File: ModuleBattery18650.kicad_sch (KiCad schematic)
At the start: 28 parts, among them J1 Connector_6p, T1 SI2323DS-T1-E3, T2 FDN337N, T3 SI2323DS-T1-E3, U1 MCP73832-2-OT, U2 MCP121T-315E

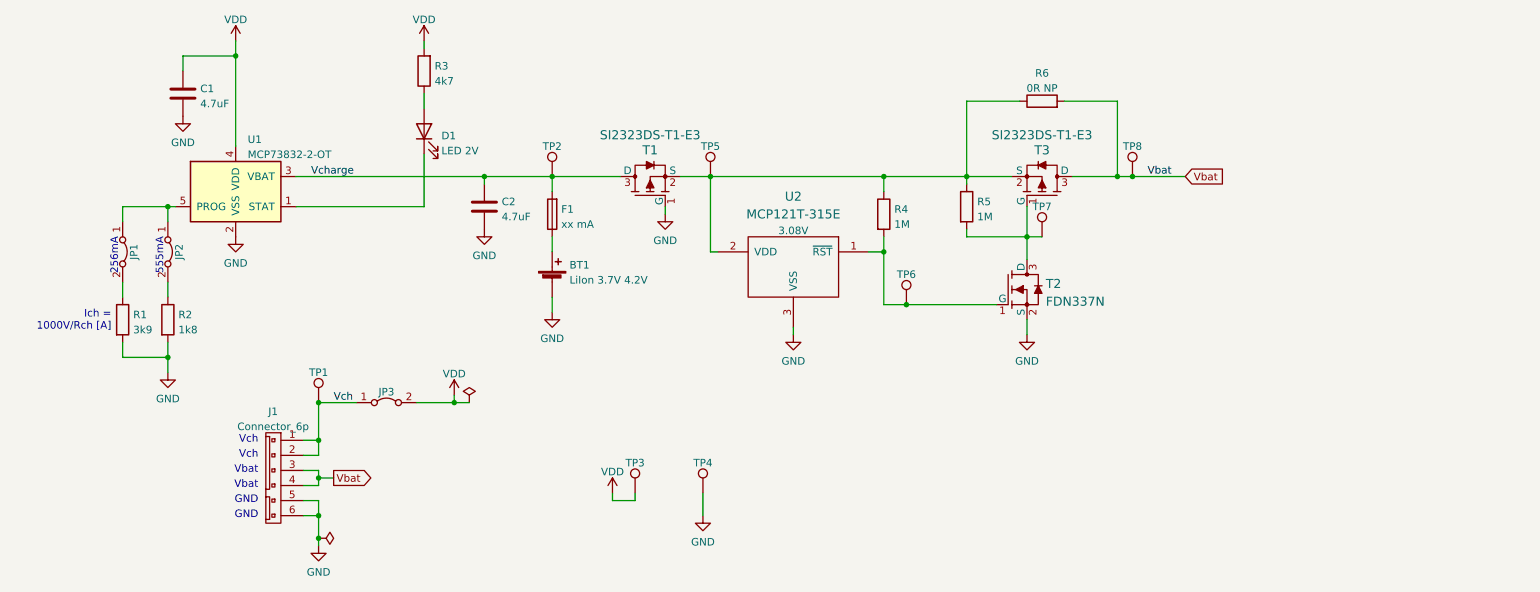
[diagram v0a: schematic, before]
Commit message: Changes
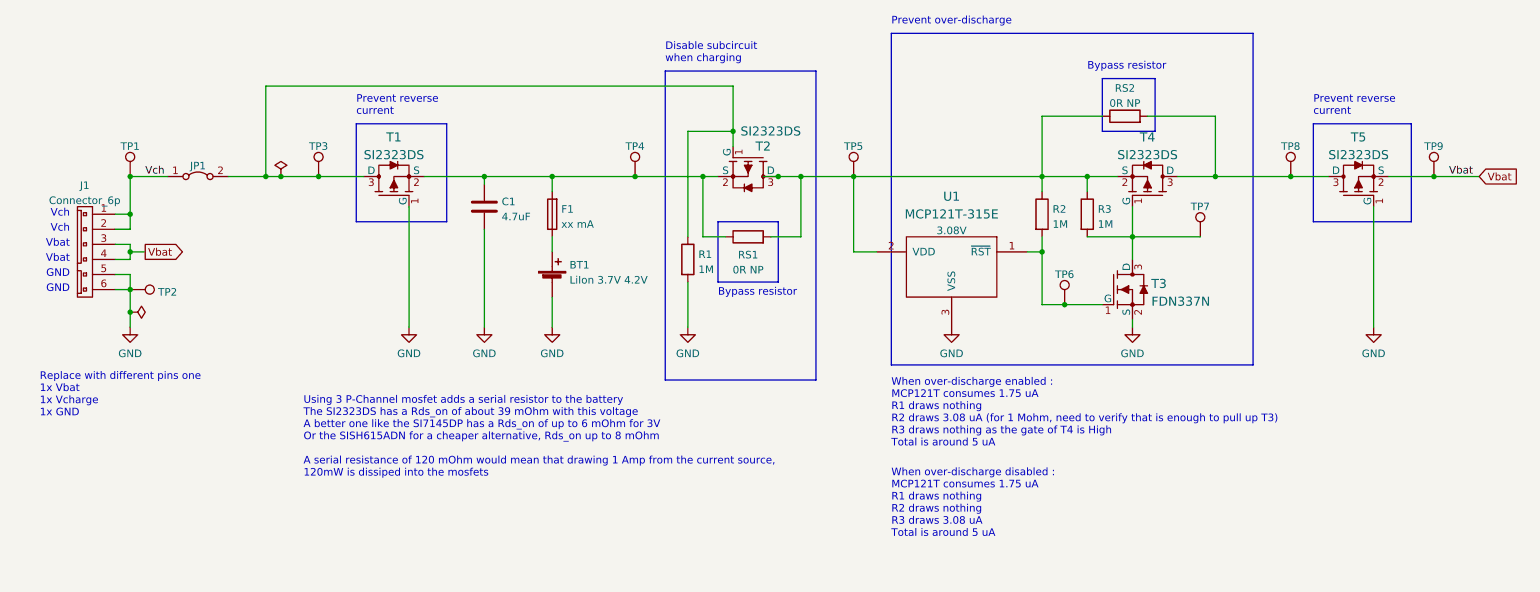
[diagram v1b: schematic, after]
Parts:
- removed C1: 4.7uF, 0ESN_Lib:C_0805_2012Metric_Pad1.18x1.45mm_HandSolder, symbol Device:C
- removed D1: LED 2V, 0ESN_Lib:D_0603_1608Metric_Pad1.05x0.95mm_HandSolder, symbol Device:LED
- removed JP1, JP2: Jumper_2_Bridged, 0ESN_Lib:PinHeader_1x02_P1.27mm_Vertical, symbol 0ESN_Lib:Jumper_2_Bridged
- removed R2: 1k8, 0ESN_Lib:R_0603_1608Metric_Pad0.98x0.95mm_HandSolder, symbol Device:R
- removed R3: 4k7, 0ESN_Lib:R_0603_1608Metric_Pad0.98x0.95mm_HandSolder, symbol Device:R
- removed U1: MCP73832-2-OT, 0ESN_Lib:SOT-23-5_HandSoldering, symbol 0ESN_Lib:MCP73832-2-OT
- added RS1: 0R NP, 0ESN_Lib:R_0603_1608Metric_Pad0.98x0.95mm_HandSolder, symbol Device:R
- added T1, T2: SI2323DS, Package_TO_SOT_SMD:SOT-23_Handsoldering, symbol 0ESN_Lib:SI2323DS
- added TP9: TestPoint, 0ESN_Lib:TestPoint_Pad_D1.0mm, symbol 0ESN_Lib:TestPoint
- R1: value 3k9 -> 1M
- T4: renamed from T3; value SI2323DS-T1-E3 -> SI2323DS; symbol 0ESN_Lib:SI2323DS-T1-E3 -> 0ESN_Lib:SI2323DS
- T5: renamed from T1; value SI2323DS-T1-E3 -> SI2323DS; symbol 0ESN_Lib:SI2323DS-T1-E3 -> 0ESN_Lib:SI2323DS
- renumbered C2 to C1, JP3 to JP1, R4 to R2, R5 to R3, R6 to RS2, T2 to T3, TP4 to TP2, TP2 to TP4, U2 to U1
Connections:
- net VDD is gone; now on an unnamed net: JP1.2 (B), TP3.1
- net GND: now also T1.1 (G)
- net Vbat: now also T5.2 (S), TP9.1; no longer RS2.2, T4.3 (D), TP8.1
- net at R2.1, R3.1, RS2.1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: now also RS1.2, T2.3 (D); no longer T5.2 (S)
- net at R1.1: now also T1.3 (D), T2.1 (G)
- net Vcharge: no longer names the net of C1.1, F1.2, TP4.1
- net Vcharge: now also RS1.1, T1.2 (S), T2.2 (S); no longer T5.3 (D)
- new net: RS2.2, T4.3 (D), T5.3 (D), TP8.1
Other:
- note added: "Bypass resistor"
- note added: "Disable subcircuit when charging"
- note added: "Prevent over-discharge"
- note added: "Prevent reverse current"
- note added: "Replace with different pins one 1x Vbat 1x Vcharge 1x GND"
- note added: "Using 3 P-Channel mosfet adds a serial resistor to the battery The SI2323DS has a Rds_on of about 39 mOhm with this voltage A better one like the SI7145DP has a Rds_on of up to 6 mOhm for 3V Or the SISH615ADN for a cheaper alternative, Rds_on up to 8 mOhm A serial resistance of 120 mOhm would mean that drawing 1 Amp from the current source, 120mW is dissiped into the mosfets"
- note added: "When over-discharge disabled : MCP121T consumes 1.75 uA R1 draws nothing R2 draws nothing R3 draws 3.08 uA Total is around 5 uA"
- note added: "When over-discharge enabled : MCP121T consumes 1.75 uA R1 draws nothing R2 draws 3.08 uA (for 1 Mohm, need to verify that is enough to pull up T3) R3 draws nothing as the gate of T4 is High Total is around 5 uA"
- note removed: "256mA"
- note removed: "555mA"
- note removed: "Ich = 1000V/Rch [A]"
- moved on the sheet: J1, JP1, R2, R3, RS2, T3, T4, T5, TP1, TP2, TP3, TP4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
